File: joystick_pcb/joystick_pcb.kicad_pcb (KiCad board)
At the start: 2 copper layers, 30 x 30 mm, 7 parts, among them J1 Conn_01x06_Pin, J2 Conn_01x06_Pin, U1 RKJXV122400R

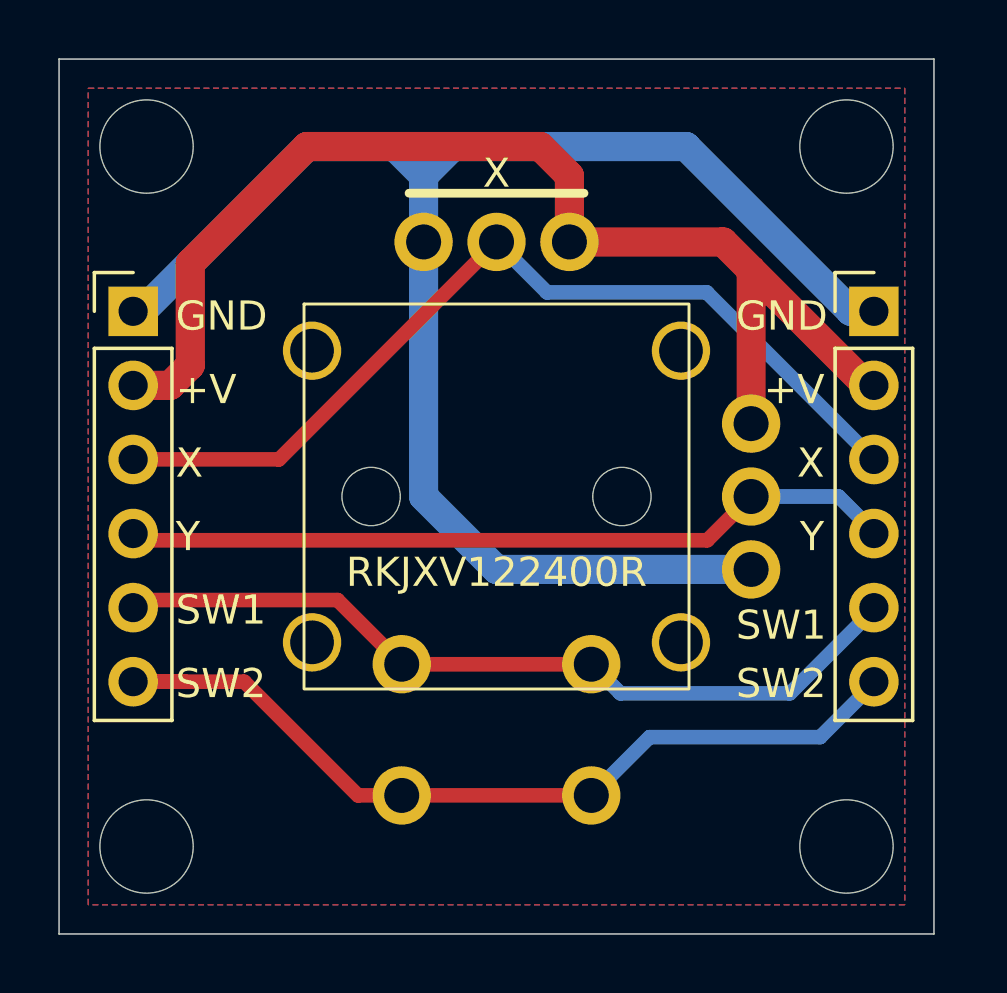
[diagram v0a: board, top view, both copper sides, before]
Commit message: updated
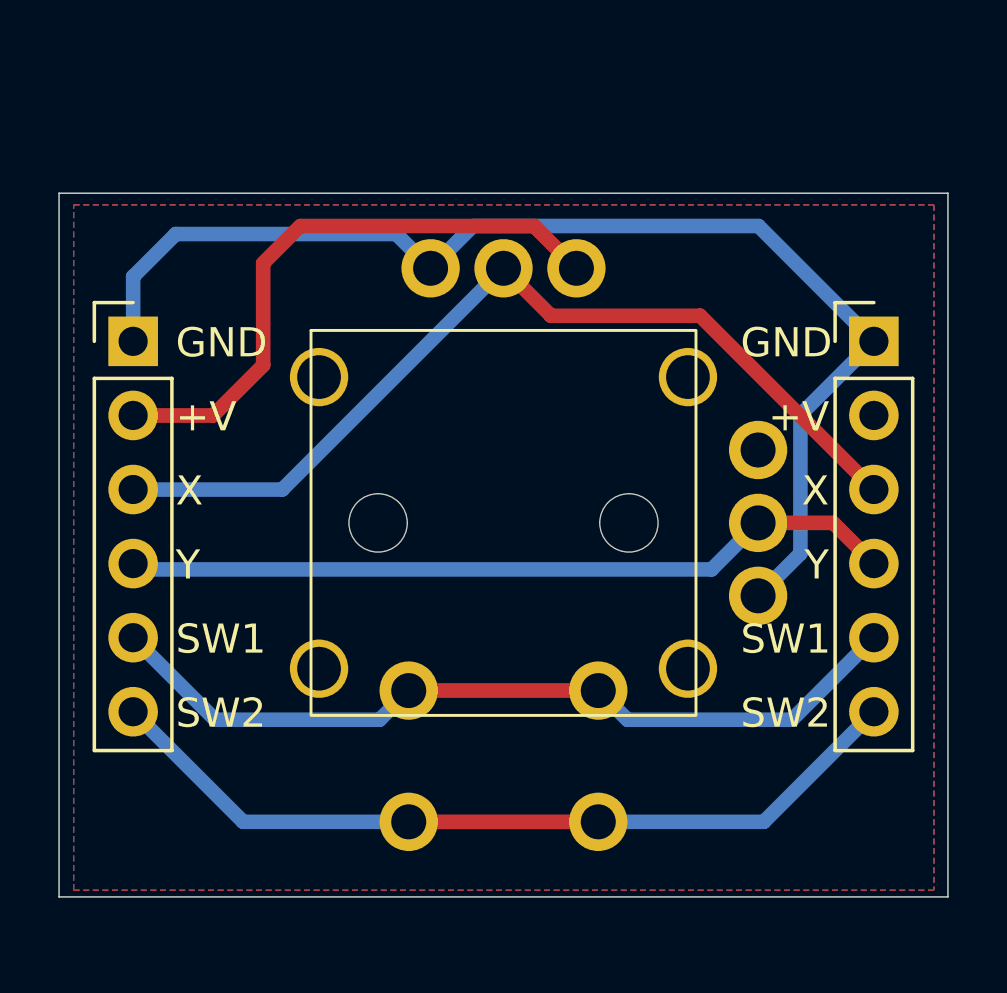
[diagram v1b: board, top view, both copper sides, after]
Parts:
- removed REF** (x4): MountingHole_3.2mm_M3, MountingHole:MountingHole_3.2mm_M3
- moved J1 1.03 mm to (22.5, 29.7)
- moved J2 1.03 mm to (47.9, 29.7)
- moved U1 0.94 mm to (35.2, 35.9)
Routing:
- net VCC: track 40.9 -> 20.5 mm
- net GND: track 54.2 -> 41.5 mm
- net SW2: track 31.0 -> 28.5 mm
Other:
- board size 30 x 30 mm -> 30.5 x 24.1 mm
